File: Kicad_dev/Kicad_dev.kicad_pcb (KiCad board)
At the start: 2 copper layers, 66 parts, among them J1 Conn_01x02_Pin, J10 Screw_Terminal_01x05_2.54mm, J2 Conn_01x02_Pin, J3 Conn_01x02_Pin, J4 530470510_Picoblade, J5 Connecteur_SMA, J6 BNC, J7 Screw_Terminal_01x02_2.54mm, J8 Screw_Terminal_01x03_2.54mm, J9 Screw_Terminal_01x04_2.54mm, Q1 IRF540N, Q2 2N7000_THT, Q3 2N7002, SW1 RotaryEncoder_Switch, SW2 RotaryEncoder_Switch, SW3 SW_DPST_x2, SW4 SW_DPST_x2, U1 COM-09032, U11 MAX-8Q, U12 LM317_TO-220, U13 LM7805_TO220, U14 DHT11, U15 DHT11, U17 ATmega328-A, U18 ATmega328-P, U19 STM32F030CCTx, U2 LM317_SOT-223, U20 STM32F446VETx, U21 STM32F723ZETx, U22 MPU-6050, U23 DS1307+, U24 DS3231M, U25 LM358, U26 TP4056, U3 74HC04, U4 L293D, U5 LM358, U6 PC817_SMD, U7 PC817_THT, U8 NEO-M8Q

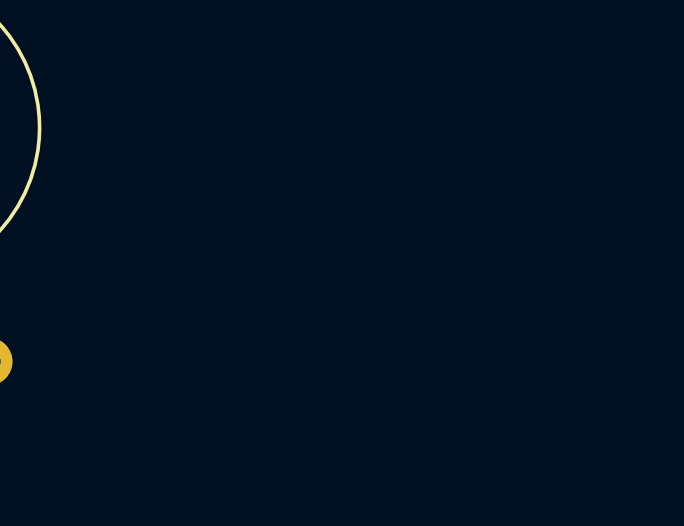
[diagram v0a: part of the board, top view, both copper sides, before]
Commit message: Add repo of lib Kicad before analyzing...
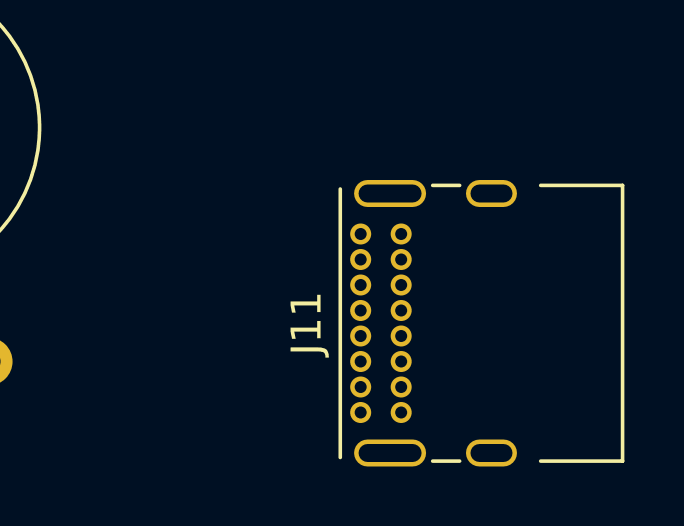
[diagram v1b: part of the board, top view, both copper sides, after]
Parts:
- added J11: USB_C_Receptacle, CREPP_Connectors_USB:USB_C_Receptacle_GCT_USB4085, F.Cu at (160.2, 155.4)
- added SERVO_SG2: ~, CREPP_Servo:SG90_Servo, F.Cu at (163.1, 122.7)
